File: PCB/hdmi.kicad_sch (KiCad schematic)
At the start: 25 parts, among them J7 HDMI_D_1.4, U12 PCA9306DC1, U14 UCL0524P, U15 UCL0524P, U16 UCL0524P

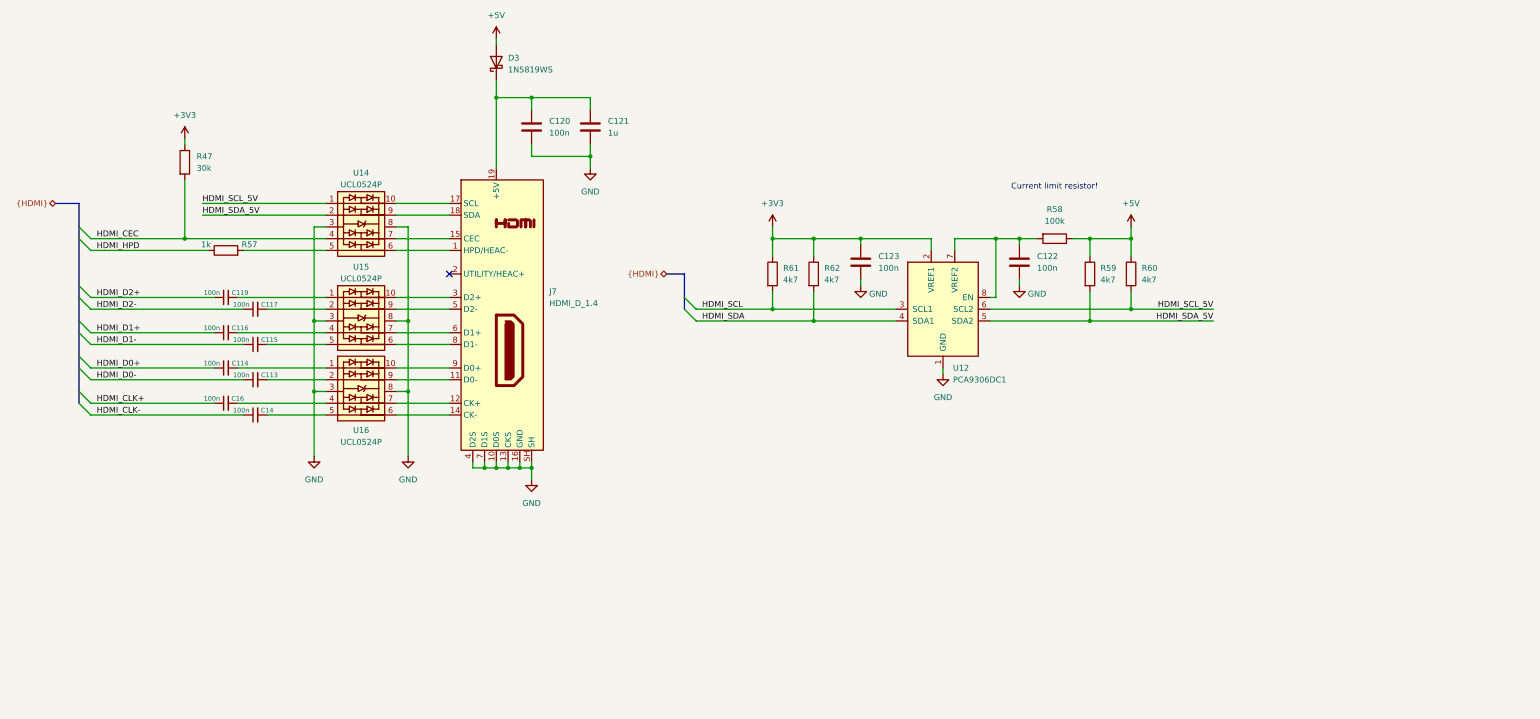
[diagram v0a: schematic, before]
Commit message: more HDMI routing
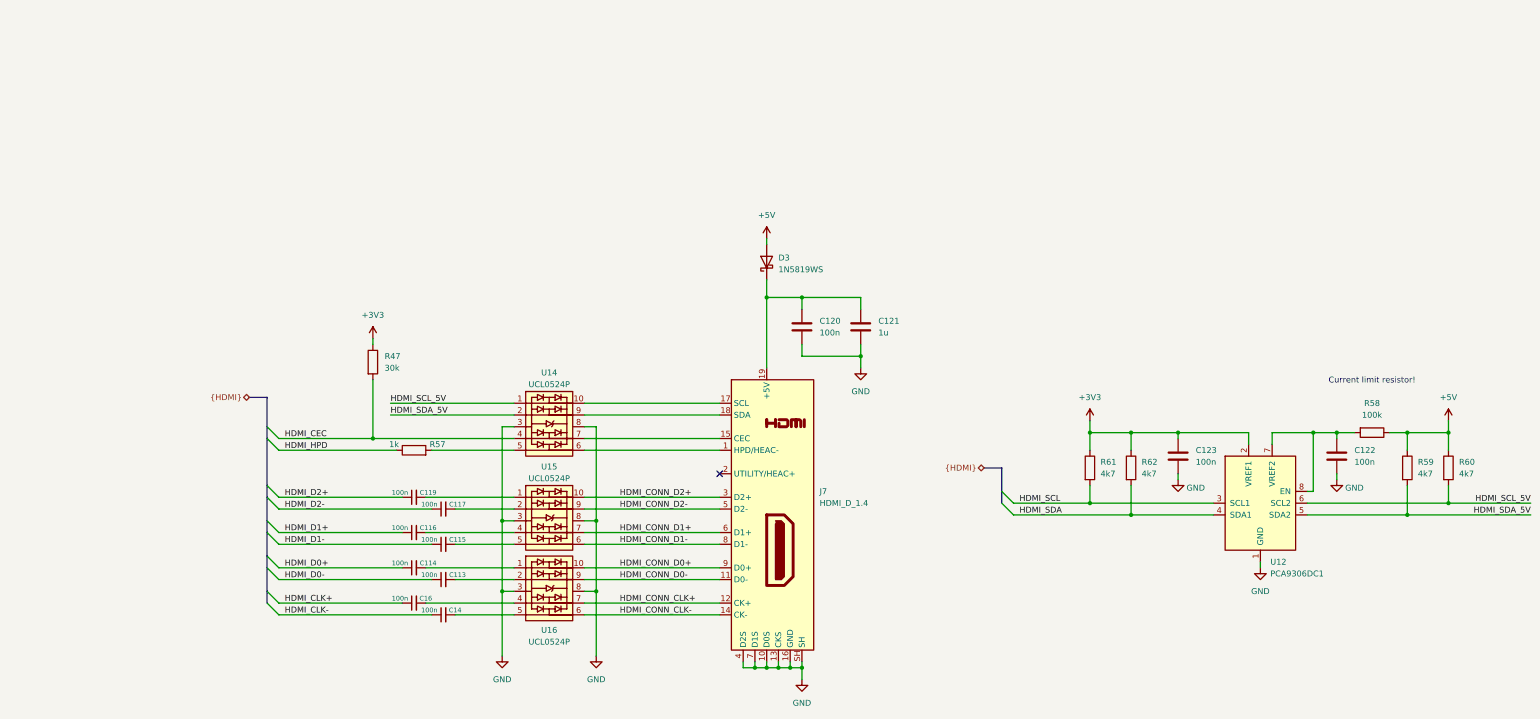
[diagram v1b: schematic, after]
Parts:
- J7: footprint Connector_Video:HDMI_Micro-D_Molex_46765-1xxx -> FPGA:Kai's_HDMI_Micro-D_Molex_46765-1xxx
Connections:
- net HDMI_CONN_D0-: now reaches J7.11 (D0-), U16.9
- net HDMI_CONN_CLK+: now reaches J7.12 (CK+), U16.7
- net HDMI_CONN_CLK-: now reaches J7.14 (CK-), U16.6
- net HDMI_CONN_D2+: now reaches J7.3 (D2+), U15.10
- net HDMI_CONN_D2-: now reaches J7.5 (D2-), U15.9
- net HDMI_CONN_D1+: now reaches J7.6 (D1+), U15.7
- net HDMI_CONN_D1-: now reaches J7.8 (D1-), U15.6
- net HDMI_CONN_D0+: now reaches J7.9 (D0+), U16.10
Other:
- moved on the sheet: C113, C114, C115, C116, C117, C119, C120, C121, C122, C123, C14, C16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
